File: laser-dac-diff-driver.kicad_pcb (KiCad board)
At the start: 2 copper layers, 52 parts, among them IC401 DCDC-CONV_TRACO_TMH-XXXX_Dual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, P101 CONN_2, P102 CONN_3X2, P103 CONN_6X2, U101 AD5689RARUZ, U102 74HC04, U201 OP470, U202 LM358, U401 LM317EMP, U402 LM317EMP, U403 LM337IMP

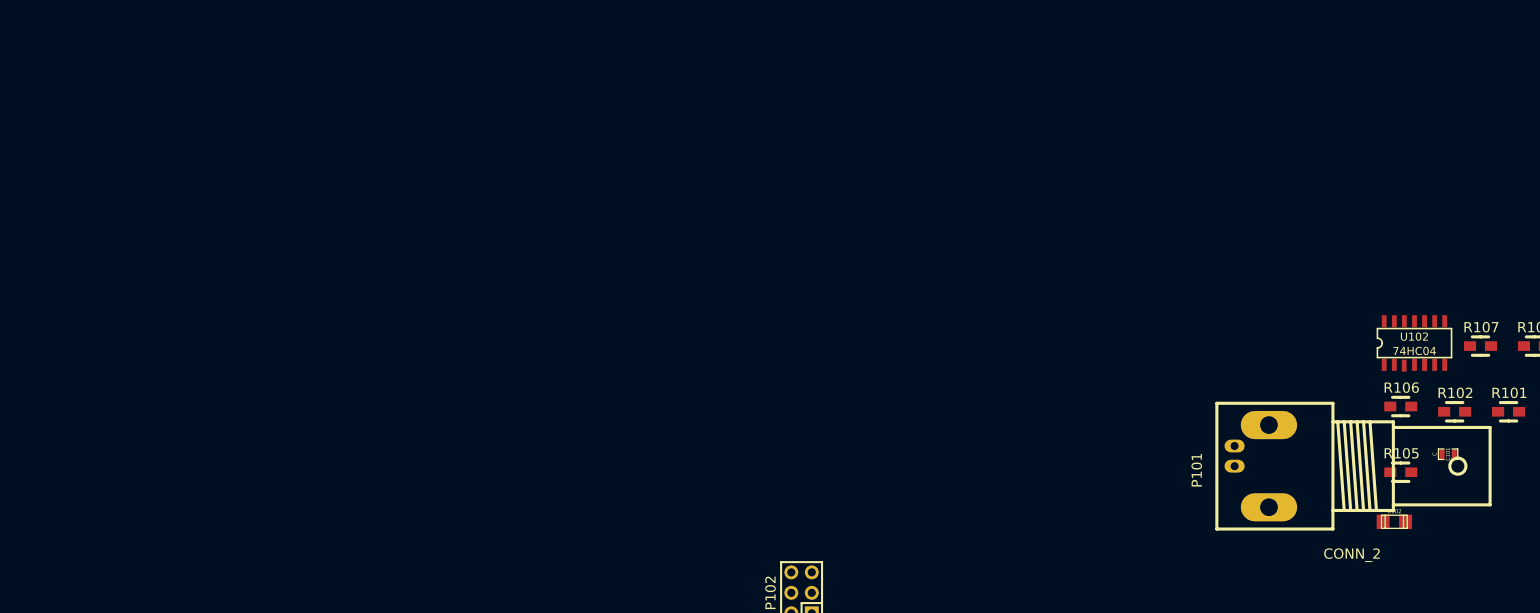
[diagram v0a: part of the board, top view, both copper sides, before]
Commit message: Moved that thing over there
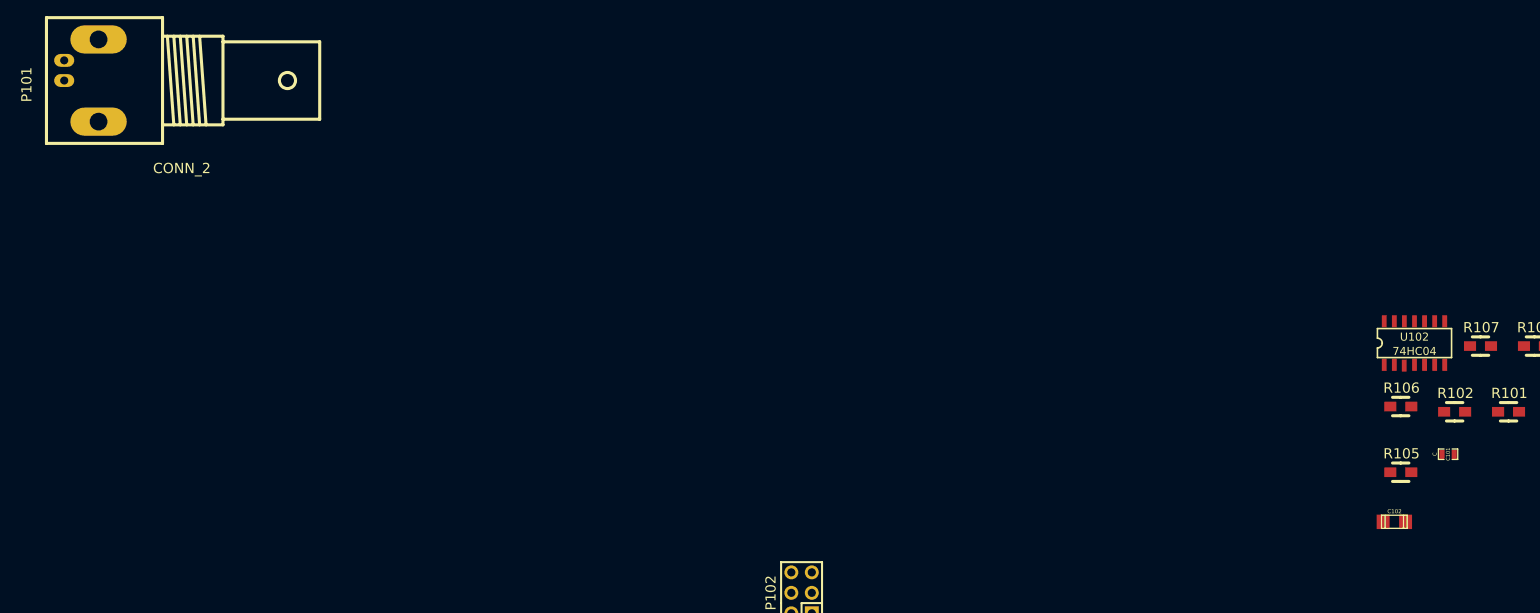
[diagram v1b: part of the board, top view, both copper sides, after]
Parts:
- moved P101 152.9 mm to (36.8, 31.8)
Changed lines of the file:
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@@
-(kicad_pcb (version 3) (host pcbnew "(2014-01-30 BZR 4648)-product")
+(kicad_pcb (version 3) (host pcbnew "(2014-02-24 BZR 4719)-product")
   (general
     (links 128)
     (no_connects 121)
-    (area 0 0 0 0)
+    (area 97.375133 52.451 288.960587 128.0244)
     (thickness 1.6)
     (drawings 0)
@@
     (pad_to_mask_clearance 0.2)
     (aux_axis_origin 0 0)
-    (visible_elements FFFFFF7F)
+    (visible_elements 7FFFFFFF)
     (pcbplotparams
       (layerselection 3178497)
@@
   )
   (module Sockets_BNC:BNC_Socket_TYCO-AMP_LargePads (layer F.Cu)
-    (at 182.044341 79.595981 270)
+    (at 36.83 31.75 270)
     (descr "BNC Socket TYCO AMP")
     (tags "BNC Socket TYCO AMP")
